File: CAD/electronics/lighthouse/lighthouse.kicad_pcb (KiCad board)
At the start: 2 copper layers, 30.5 x 23.5 mm, 12 parts, among them J1 Battery, J2 LED, J3 DC Motor, Q1 Q_NPN_Darlington_EBC, SW1 Tilt switch

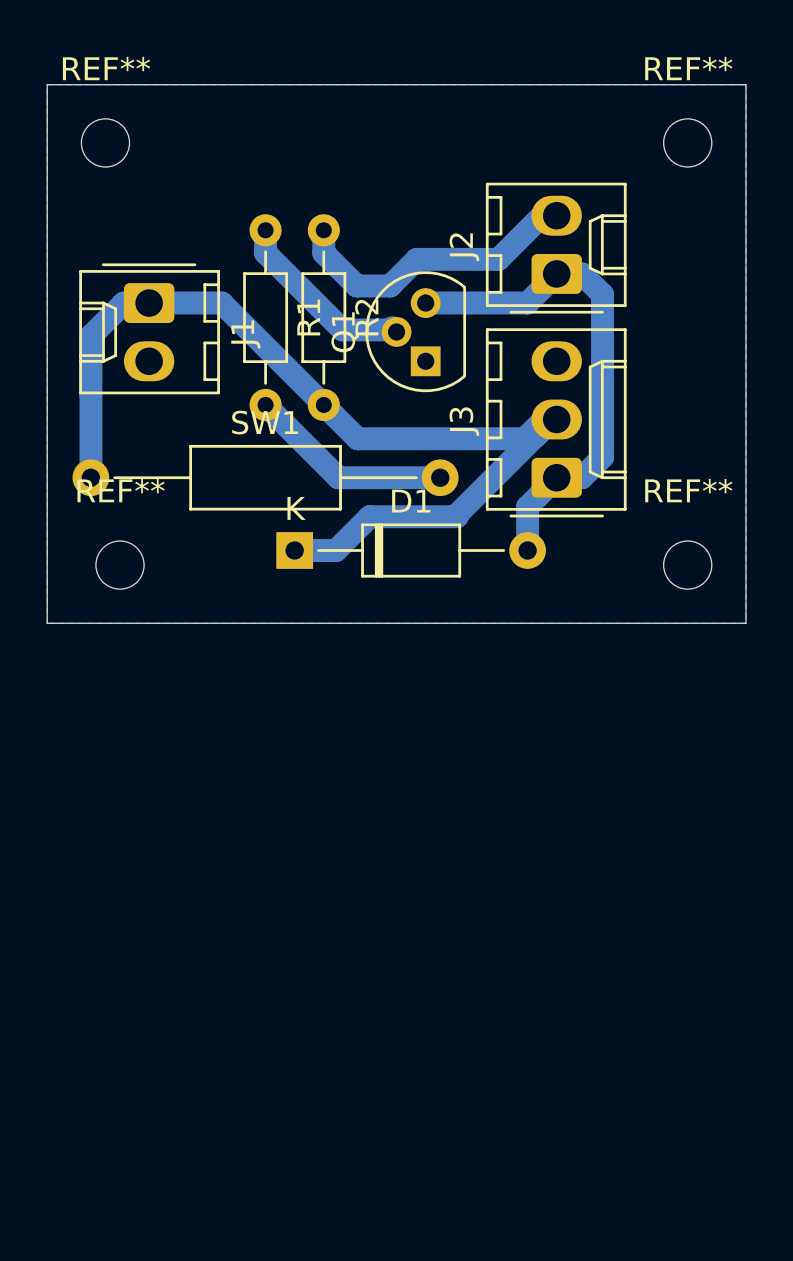
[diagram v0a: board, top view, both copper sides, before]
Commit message: Electronics sent to manufacturer
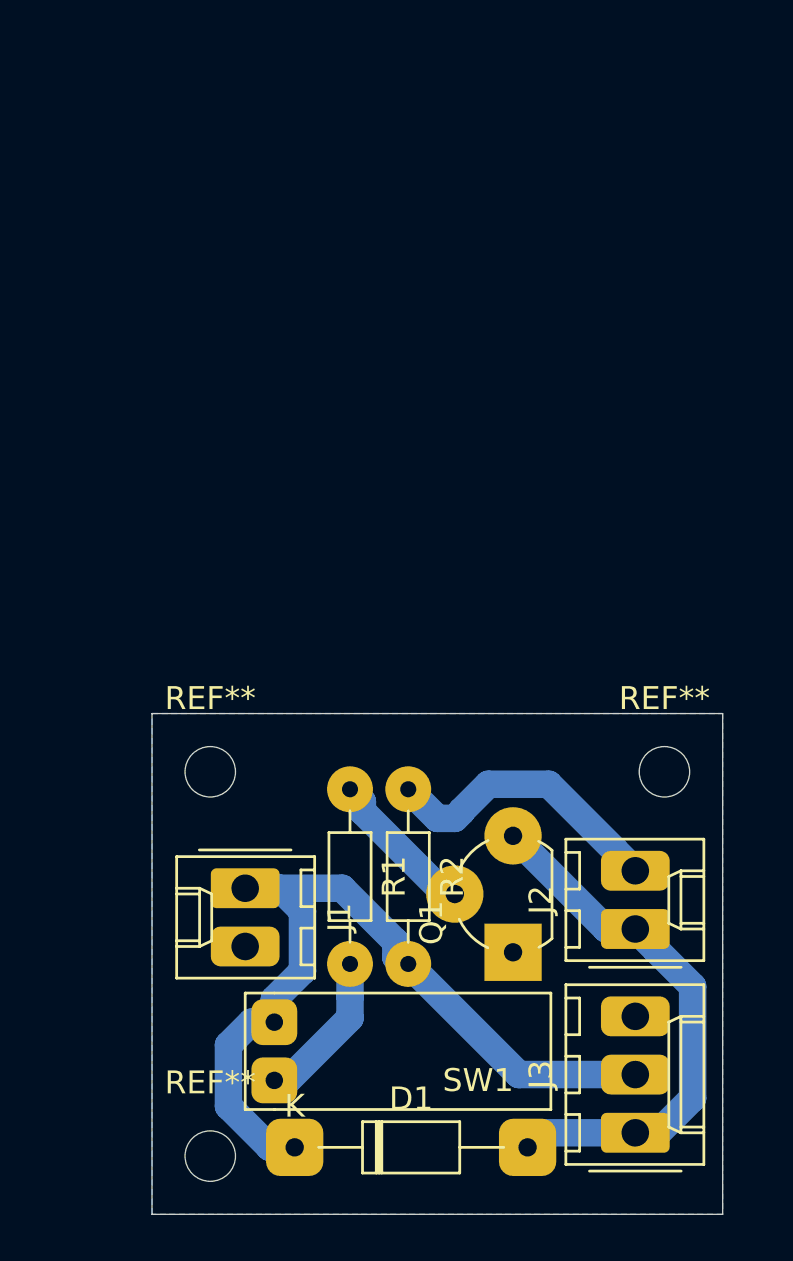
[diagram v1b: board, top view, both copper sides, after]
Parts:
- removed the REF** at (80.0, 67.3)
- removed the REF** at (55.2, 67.3)
- removed the REF** at (54.6, 48.9)
- removed the REF** at (80.0, 48.9)
- added REF**: MountingHole_2.2mm_M2, MountingHole:MountingHole_2.2mm_M2, F.Cu at (79.0, 76.3)
- added REF**: MountingHole_2.2mm_M2, MountingHole:MountingHole_2.2mm_M2, F.Cu at (59.2, 93.1)
- added REF**: MountingHole_2.2mm_M2, MountingHole:MountingHole_2.2mm_M2, F.Cu at (59.2, 76.3)
- Q1: footprint Package_TO_SOT_THT:TO-92L -> Package_TO_SOT_THT:TO-92L_Wide
- SW1: footprint Resistor_THT:R_Axial_DIN0207_L6.3mm_D2.5mm_P15.24mm_Horizontal -> lighthouse:Mercury tilt switch
- moved J2 28.8 mm to (77.7, 83.2)
- moved J3 28.8 mm to (77.7, 92.1)
- moved Q1 26.1 mm to (72.4, 84.2)
- moved D1 26.0 mm to (62.9, 92.7)
- moved J1 25.9 mm to (60.7, 81.4)
- moved SW1 25.1 mm to (62.0, 87.2)
- moved R1 24.7 mm to (65.3, 77.1)
- moved R2 24.7 mm to (67.8, 77.1)
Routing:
- net Net-(D1-Pad1): track 45.0 -> 36.3 mm
- net Net-(R1-Pad2): track 8.94 -> 6.79 mm
- net Net-(D1-Pad2): track 21.8 -> 23.5 mm
- net Net-(Q1-Pad2): track 7.95 -> 6.71 mm
- net Net-(J2-Pad2): track 13.6 -> 12.6 mm
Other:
- board size 30.5 x 23.5 mm -> 24.9 x 21.8 mm
- net class Default: trace_width 1 -> 1.2
